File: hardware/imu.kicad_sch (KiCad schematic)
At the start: 1 part, among them U601 LSM6DSM

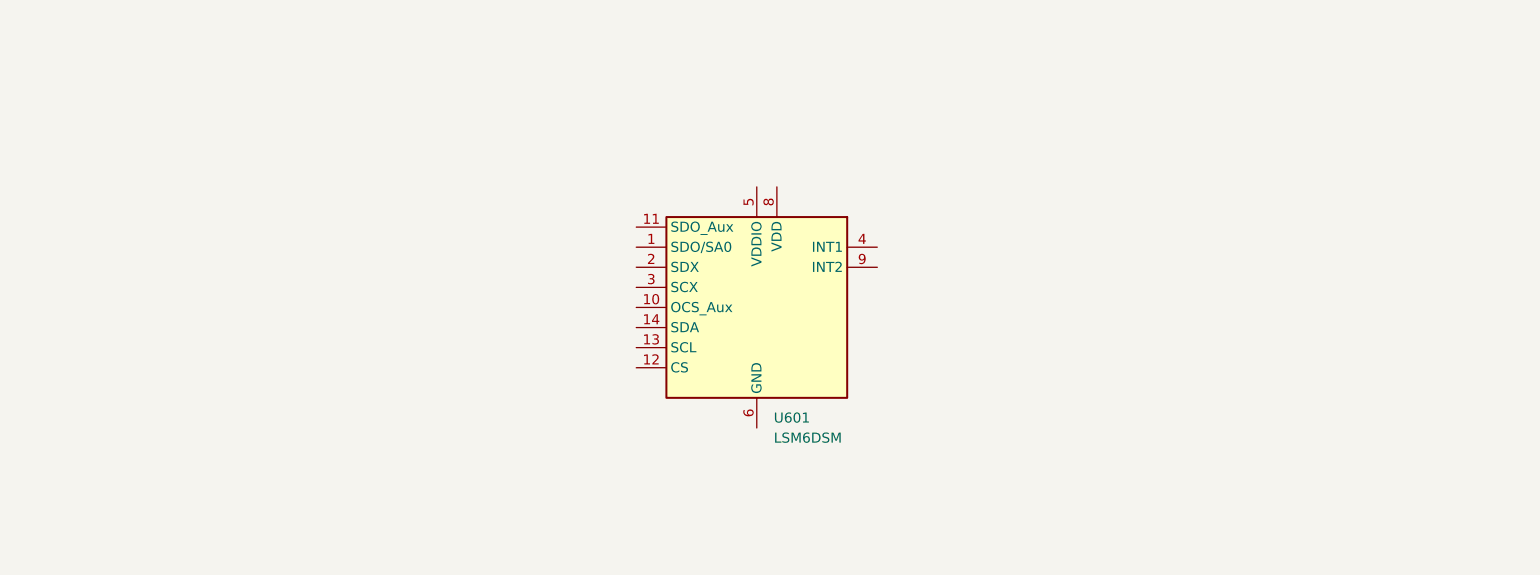
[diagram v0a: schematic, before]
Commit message: updated pcb
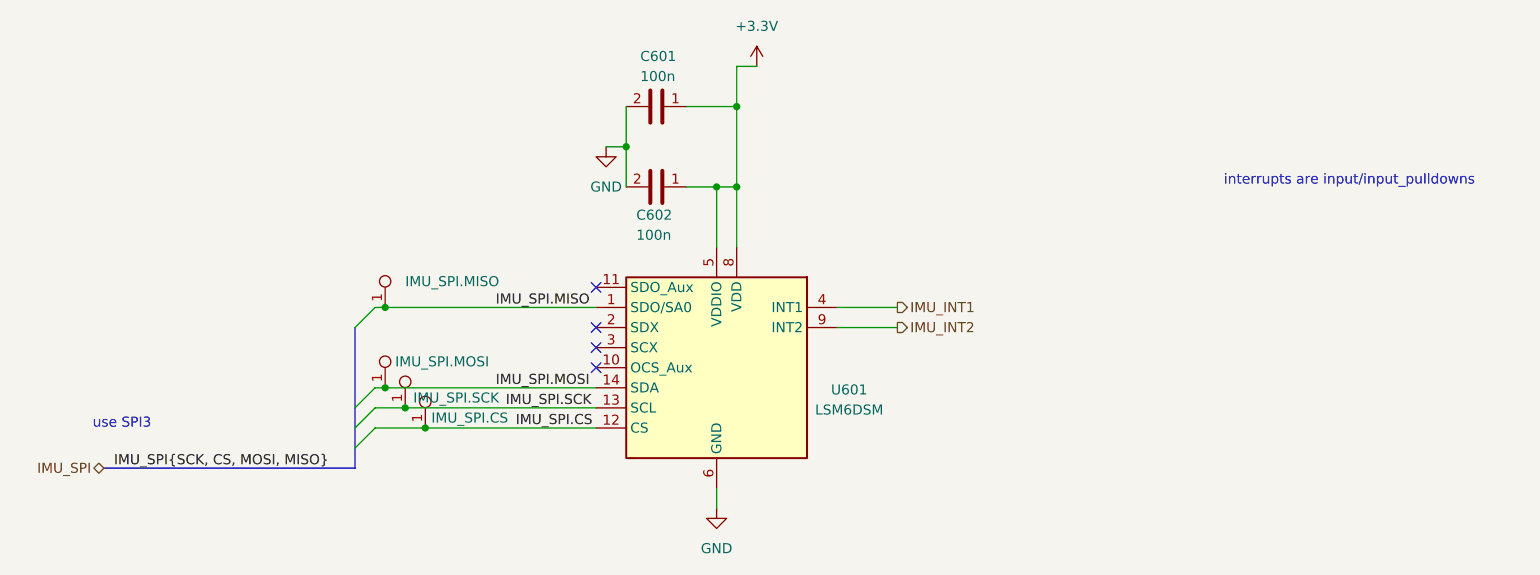
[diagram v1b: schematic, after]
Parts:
- added C601, C602: 100n, Capacitor_SMD:C_0603_1608Metric_Pad1.08x0.95mm_HandSolder, symbol bfr_capacitors:06035C104KAT2A
- added TP601: IMU_SPI.MISO, bfr_utilities:TestPoint_Keystone_5019_Miniature, symbol bfr_master:SMD_Test_Point
- added TP602: IMU_SPI.MOSI, bfr_utilities:TestPoint_Keystone_5019_Miniature, symbol bfr_master:SMD_Test_Point
- added TP603: IMU_SPI.SCK, bfr_utilities:TestPoint_Keystone_5019_Miniature, symbol bfr_master:SMD_Test_Point
- added TP604: IMU_SPI.CS, bfr_utilities:TestPoint_Keystone_5019_Miniature, symbol bfr_master:SMD_Test_Point
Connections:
- net IMU_SPI.MISO: now reaches U601.1 (SDO/SA0)
- net IMU_SPI.MISO: now also TP601.1
- net IMU_SPI.CS: now reaches U601.12 (CS)
- net IMU_SPI.CS: now also TP604.1
- net IMU_SPI.SCK: now reaches U601.13 (SCL)
- net IMU_SPI.SCK: now also TP603.1
- net IMU_SPI.MOSI: now reaches U601.14 (SDA)
- net IMU_SPI.MOSI: now also TP602.1
- net IMU_INT1: now reaches U601.4 (INT1)
- net +3.3V: now reaches U601.5 (VDDIO)
- net +3.3V: now also U601.8 (VDD), C601.1, C602.1
- net GND: now reaches U601.6 (GND), U601.7 (GND)
- net GND: now also C601.2, C602.2
- net IMU_INT2: now reaches U601.9 (INT2)
- no-connect marks 0 -> 4
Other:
- note added: "interrupts are input/input_pulldowns"
- note added: "use SPI3"
- moved on the sheet: U601
